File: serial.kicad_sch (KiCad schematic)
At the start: 11 parts, among them J301 USB_B_Micro, U301 XC6206P332MR, U302 CH340N, U303 USBLC6-2SC6

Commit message: Rework parts and order informations
Signed-off-by: Benedikt Spranger <b.spranger@linutronix.de>
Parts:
- C301, C302: footprint (none) -> Capacitor_SMD:C_0603_1608Metric; LCSC# (none) -> C15849; Manufacture (none) -> Samsung Electro-Mechanics; assemble (none) -> y; mpn (none) -> CL10A105KB8NNNC
- C303, C304: footprint (none) -> Capacitor_SMD:C_0402_1005Metric; LCSC# (none) -> C307331; Manufacture (none) -> Samsung Electro-Mechanics; assemble (none) -> y; mpn (none) -> CL05B104KB54PNC
- D301: footprint (none) -> LED_SMD:LED_0603_1608Metric; LCSC# (none) -> C2286; Manufacture (none) -> Hubei KENTO Elec; assemble (none) -> y; mpn (none) -> KT-0603R
- FB301: footprint (none) -> Inductor_SMD:L_0603_1608Metric; LCSC# (none) -> C1002; Manufacture (none) -> Sunlord; assemble (none) -> y; mpn (none) -> GZ1608D601TF
- J301: footprint (none) -> Connector_USB:USB_Micro-B_Amphenol_10118193-0001LF_Horizontal; LCSC# (none) -> C132563; Manufacture (none) -> Amphenol ICC; assemble (none) -> y; mpn (none) -> 10118194-0001LF
- R301: footprint (none) -> Resistor_SMD:R_0402_1005Metric; LCSC# (none) -> C11702; Manufacture (none) -> UNI-ROYAL(Uniroyal Elec); assemble (none) -> y; mpn (none) -> 0402WGF1001TCE
- U301: LCSC# (none) -> C5446; Manufacture (none) -> Torex Semicon; assemble (none) -> y; mpn (none) -> XC6206P332MR-G
- U302: LCSC# (none) -> C2977777; Manufacture (none) -> WCH(Jiangsu Qin Heng); assemble (none) -> y; mpn (none) -> CH340N
- U303: LCSC# (none) -> C2827654; Manufacture (none) -> TECH PUBLIC; assemble (none) -> y; mpn (none) -> USBLC6-2SC6

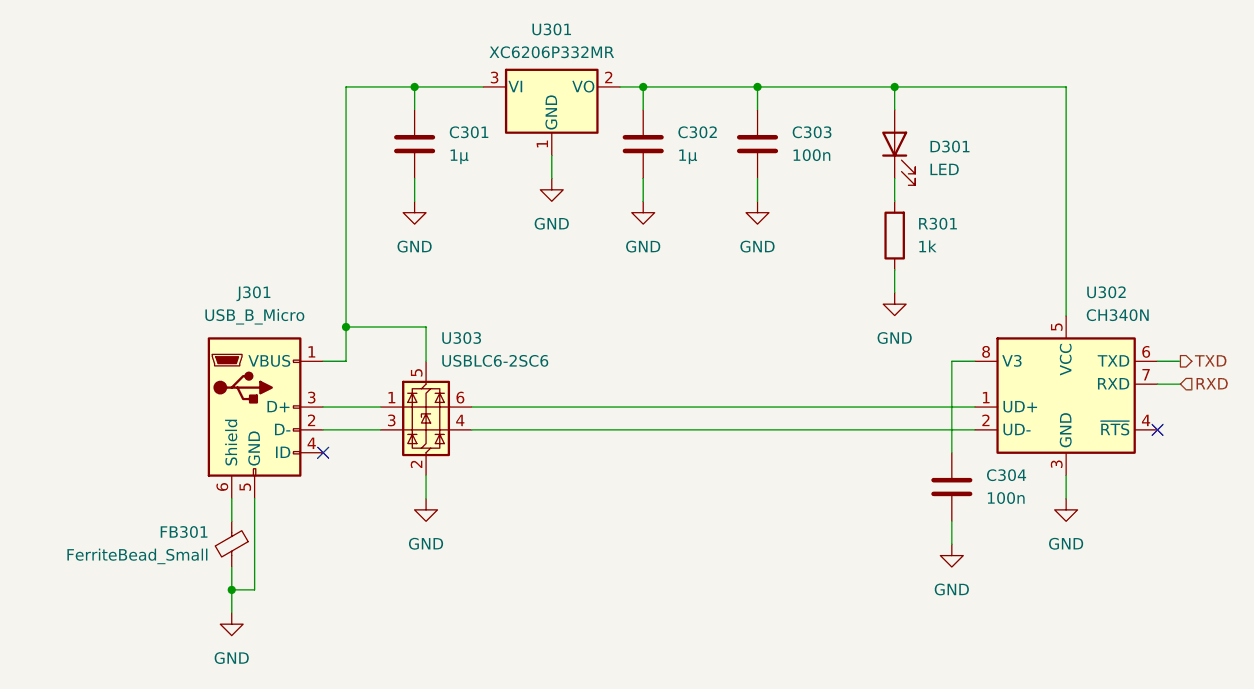
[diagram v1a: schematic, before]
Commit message: Initial layout
Signed-off-by: Benedikt Spranger <b.spranger@linutronix.de>
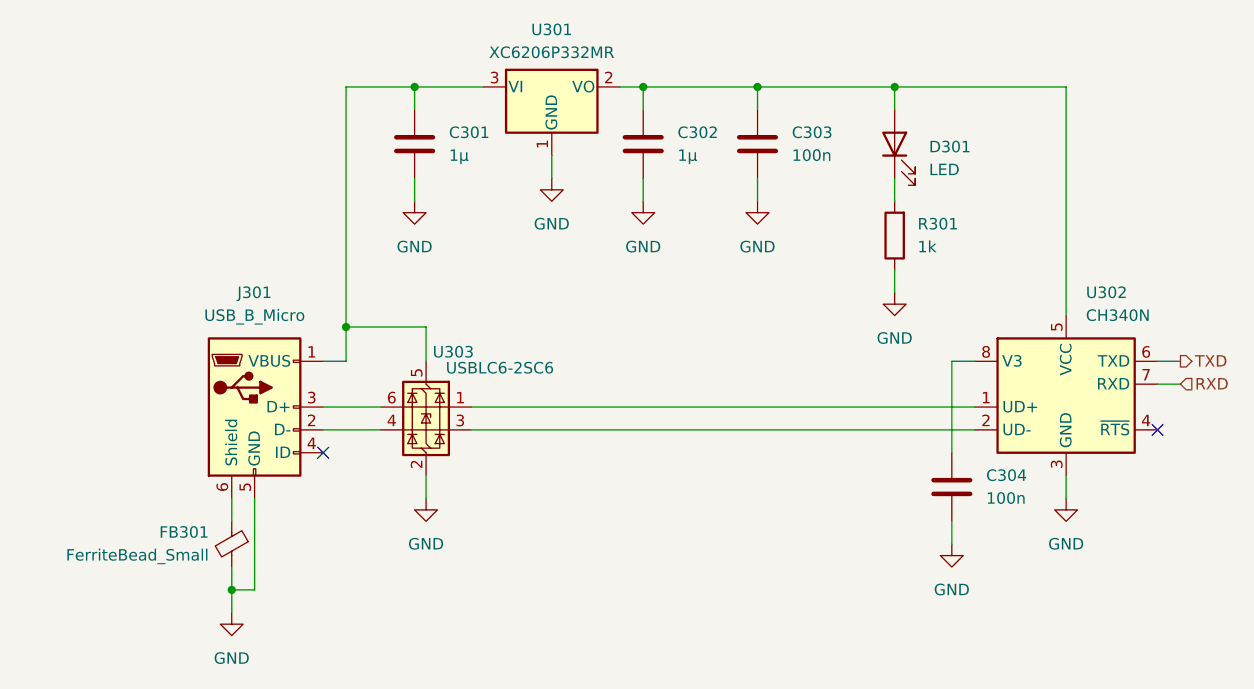
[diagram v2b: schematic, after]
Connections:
- net at U303.1 (I/O1): now also U302.1 (UD+); no longer J301.3 (D+)
- net at U303.3 (I/O2): now also U302.2 (UD-); no longer J301.2 (D-)
- net at U303.4 (I/O2): now also J301.2 (D-); no longer U302.2 (UD-)
- net at U303.6 (I/O1): now also J301.3 (D+); no longer U302.1 (UD+)
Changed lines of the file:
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@@
 		(lib_id "Power_Protection:USBLC6-2SC6")
 		(at 144.78 67.31 0)
+		(mirror y)
 		(unit 1)
 		(exclude_from_sim no)
@@
 		(on_board yes)
 		(dnp no)
-		(fields_autoplaced yes)
 		(property "Reference" "U303"
-			(at 146.4311 59.69 0)
+			(at 150.114 61.214 0)
 			(effects
 				(font
@@
 		)
 		(property "Value" "USBLC6-2SC6"
-			(at 146.4311 62.23 0)
+			(at 159.004 62.992 0)
 			(effects
 				(font
@@
 		)
 		(property "Footprint" "Package_TO_SOT_SMD:SOT-23-6"
-			(at 146.05 73.66 0)
+			(at 143.51 73.66 0)
 			(effects
 				(font
@@
 		)
 		(property "Datasheet" "https://www.st.com/resource/en/datasheet/usblc6-2.pdf"
-			(at 146.05 75.565 0)
+			(at 143.51 75.565 0)
 			(effects
 				(font

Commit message: Add legalese
Signed-off-by: Benedikt Spranger <b.spranger@linutronix.de>
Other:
- company: (none) -> Eurovibes Benedikt Spranger
- title: (none) -> DCC Licht
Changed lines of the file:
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@@
 	(paper "A4")
 	(title_block
+		(title "DCC Licht")
 		(date "2025-01-22")
 		(rev "v0.1")
+		(company "Eurovibes Benedikt Spranger")
+		(comment 1 "SPDX-License-Identifier: CERN-OHL-S-2.0")
+		(comment 2 "https://ohwr.org/cern_ohl_s_v2.txt")
+		(comment 3 "To view a copy of this license, visit")
+		(comment 4 "This work is licensed under the CERN-OHL-S v2")
 	)
 	(junction
